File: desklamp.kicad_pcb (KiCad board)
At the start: 2 copper layers, 85.1 x 35.6 mm, 13 parts, among them J1 Power, J2 Neopixel, U1 itsy_bitsy

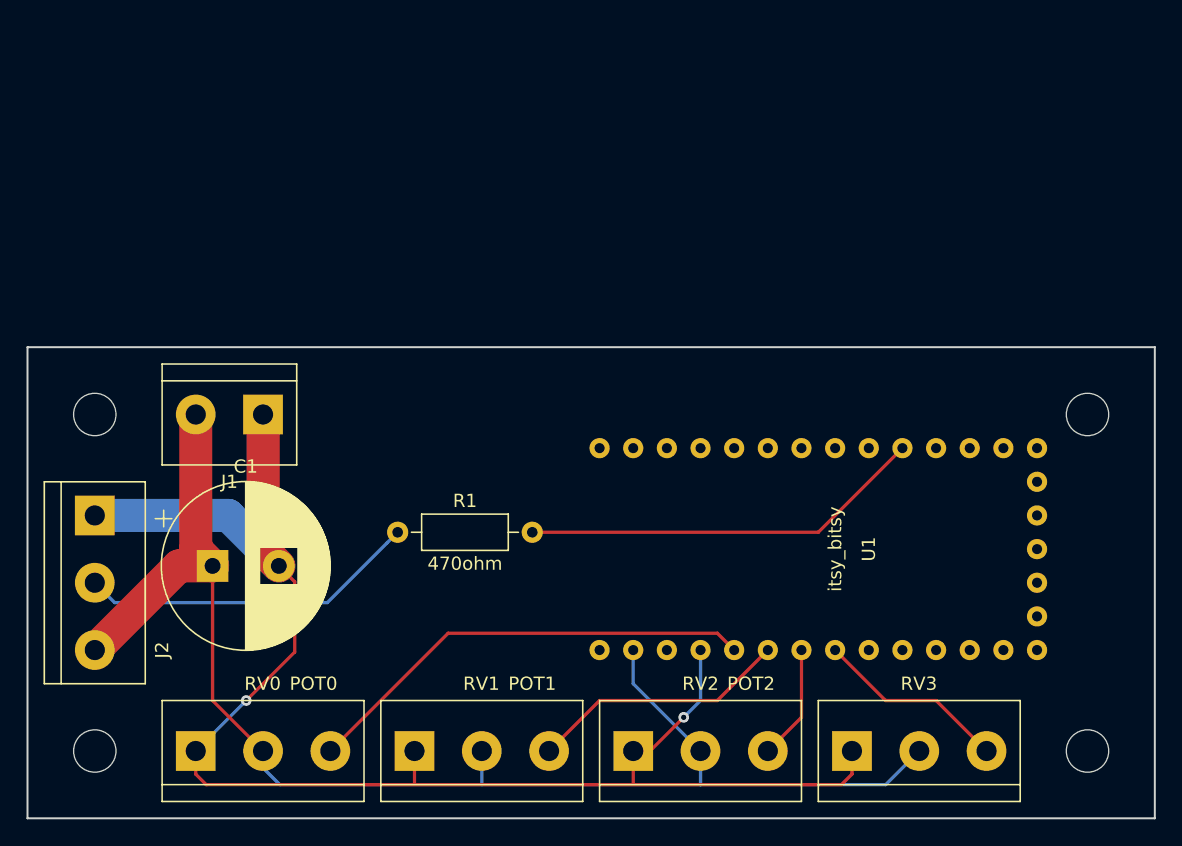
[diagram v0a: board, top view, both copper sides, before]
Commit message: Total PCB redesign
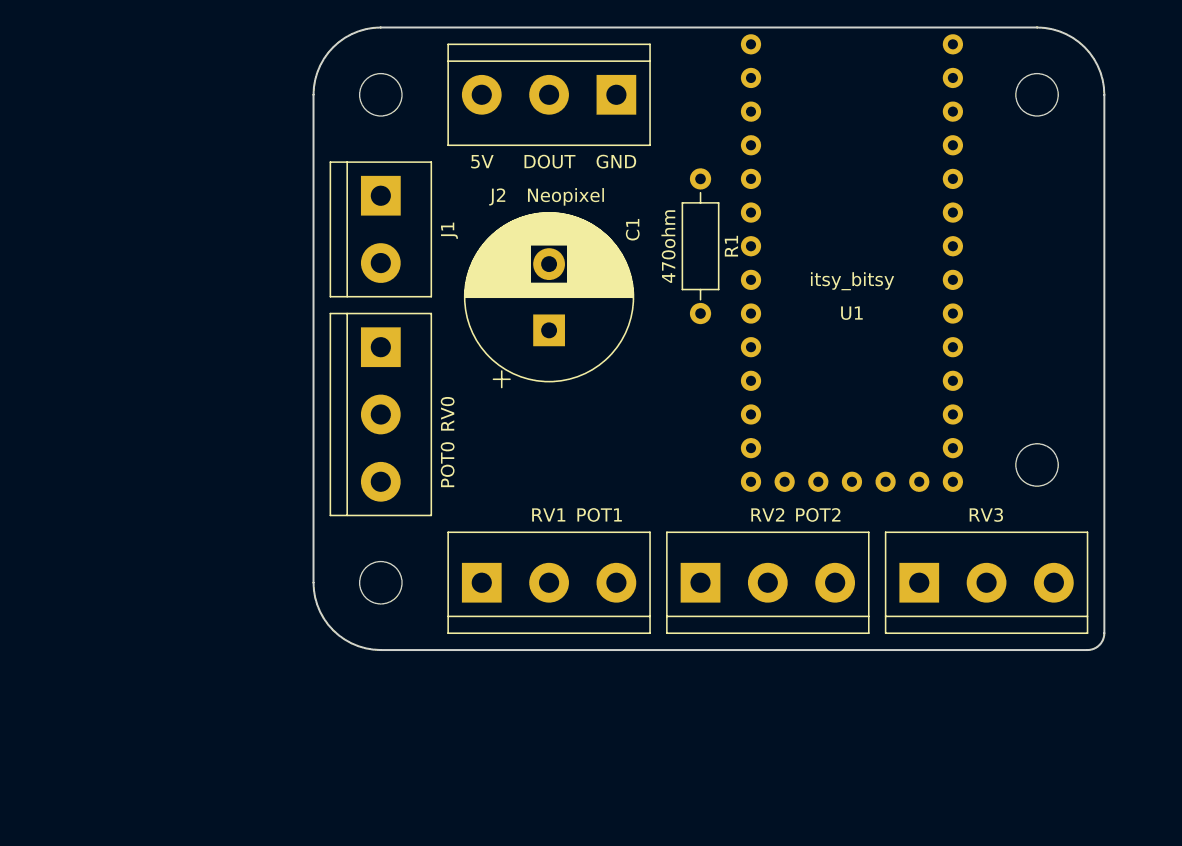
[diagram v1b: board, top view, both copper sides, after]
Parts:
- removed the REF** at (208.3, 123.2)
- removed the REF** at (208.3, 97.8)
- removed the REF** at (133.3, 97.8)
- added REF**: MountingHole_3.2mm_M3, MountingHole:MountingHole_3.2mm_M3, F.Cu at (204.5, 101.6)
- added REF**: MountingHole_3.2mm_M3, MountingHole:MountingHole_3.2mm_M3, F.Cu at (204.5, 73.7)
- added REF**: MountingHole_3.2mm_M3, MountingHole:MountingHole_3.2mm_M3, F.Cu at (154.9, 73.7)
- moved J2 50.6 mm to (172.7, 73.7), turned to 180 degrees
- moved U1 47.1 mm to (182.9, 69.8), turned to 0 degrees
- moved R1 35.1 mm to (179.1, 80.0), turned to 270 degrees
- moved RV0 33.5 mm to (154.9, 92.7), turned to 270 degrees
- moved C1 31.0 mm to (167.6, 91.4), turned to 90 degrees
- moved REF** 25.0 mm to (154.9, 110.5)
- moved J1 18.8 mm to (154.9, 81.3), turned to 270 degrees
- moved RV1 13.7 mm to (162.6, 110.5)
- moved RV3 13.7 mm to (195.6, 110.5)
- moved RV2 13.7 mm to (179.1, 110.5)
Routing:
- net GND: track 114.2 -> 0.00 mm, vias 2 -> 0
- net +5V: track 106.2 -> 0.00 mm
- net Net-(RV0-Pad3): track 34.7 -> 0.00 mm
- net Signal: track 30.6 -> 0.00 mm
- net Net-(J2-Pad2): track 25.7 -> 0.00 mm
- net Net-(RV1-Pad3): track 19.7 -> 0.00 mm
- net Net-(RV3-Pad3): track 14.6 -> 0.00 mm
- net Net-(RV2-Pad3): track 8.67 -> 0.00 mm
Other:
- board size 85.1 x 35.6 mm -> 59.7 x 47 mm
